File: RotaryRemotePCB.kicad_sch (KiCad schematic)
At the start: 10 parts, among them J1 Conn_01x02, J2 UART, J3 i2c, J4 Neopixel Connector, J5 EncoderRotary, J6 EncoderSwitch, SW1 RotaryEncoder_Switch, U1 TP4056, U2 WeMos_D1_mini

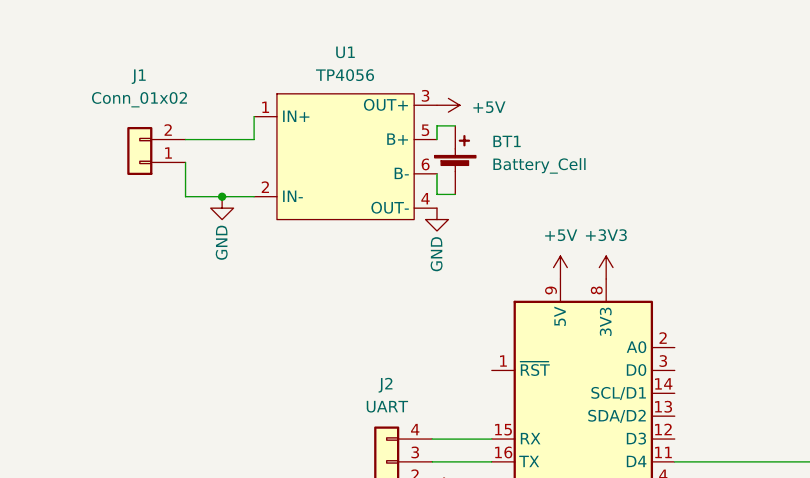
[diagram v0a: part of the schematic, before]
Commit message: Add git submodule
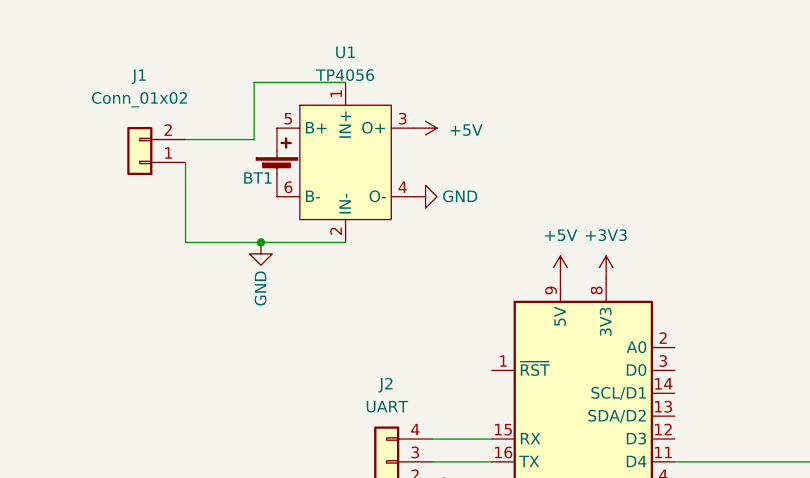
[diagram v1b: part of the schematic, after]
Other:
- moved on the sheet: BT1, U1
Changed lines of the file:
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@@
   (junction (at 205.994 86.106) (diameter 0) (color 0 0 0 0)
   )
+  (junction (at 135.128 56.642) (diameter 0) (color 0 0 0 0)
+  )
   (junction (at 230.632 86.106) (diameter 0) (color 0 0 0 0)
   )
@@
   (junction (at 230.632 91.186) (diameter 0) (color 0 0 0 0)
   )
-  (junction (at 130.81 51.562) (diameter 0) (color 0 0 0 0)
-  )
   (junction (at 205.994 91.186) (diameter 0) (color 0 0 0 0)
   )
+  (wire (pts (xy 135.128 56.642) (xy 126.746 56.642))
+    (stroke (width 0) (type default) (color 0 0 0 0))
+  )
   (wire (pts (xy 205.994 91.186) (xy 213.614 91.186))
     (stroke (width 0) (type default) (color 0 0 0 0))
@@
     (stroke (width 0) (type default) (color 0 0 0 0))
   )
-  (wire (pts (xy 154.686 43.688) (xy 156.718 43.688))
-    (stroke (width 0) (type default) (color 0 0 0 0))
-  )
   (wire (pts (xy 205.994 86.106) (xy 213.614 86.106))
     (stroke (width 0) (type default) (color 0 0 0 0))
@@
     (stroke (width 0) (type default) (color 0 0 0 0))
   )
-  (wire (pts (xy 126.746 51.562) (xy 126.746 47.752))
-    (stroke (width 0) (type default) (color 0 0 0 0))
-  )
   (wire (pts (xy 154.178 78.486) (xy 160.782 78.486))
     (stroke (width 0) (type default) (color 0 0 0 0))
@@
     (stroke (width 0) (type default) (color 0 0 0 0))
   )
-  (wire (pts (xy 154.686 49.022) (xy 154.686 51.308))
-    (stroke (width 0) (type default) (color 0 0 0 0))
-  )
-  (wire (pts (xy 154.686 45.212) (xy 154.686 43.688))
-    (stroke (width 0) (type default) (color 0 0 0 0))
-  )
   (wire (pts (xy 228.854 86.106) (xy 230.632 86.106))
     (stroke (width 0) (type default) (color 0 0 0 0))
@@
     (stroke (width 0) (type default) (color 0 0 0 0))
   )
-  (wire (pts (xy 134.366 45.212) (xy 134.366 42.672))
+  (wire (pts (xy 134.366 38.862) (xy 134.366 45.212))
     (stroke (width 0) (type default) (color 0 0 0 0))
   )
@@
     (stroke (width 0) (type default) (color 0 0 0 0))
   )
-  (wire (pts (xy 154.686 51.308) (xy 156.718 51.308))
+  (wire (pts (xy 144.526 38.862) (xy 134.366 38.862))
     (stroke (width 0) (type default) (color 0 0 0 0))
   )
@@
     (stroke (width 0) (type default) (color 0 0 0 0))
   )
-  (wire (pts (xy 134.366 51.562) (xy 130.81 51.562))
-    (stroke (width 0) (type default) (color 0 0 0 0))
-  )
-  (wire (pts (xy 130.81 51.562) (xy 126.746 51.562))
+  (wire (pts (xy 144.526 56.642) (xy 135.128 56.642))
+    (stroke (width 0) (type default) (color 0 0 0 0))
+  )
+  (wire (pts (xy 126.746 47.752) (xy 126.746 56.642))
     (stroke (width 0) (type default) (color 0 0 0 0))
   )
@@
     )
   )
-  (symbol (lib_id "power:GND") (at 130.81 51.562 0) (unit 1)
-    (in_bom yes) (on_board yes)
-    (property "Reference" "#PWR0101" (id 0) (at 130.81 57.912 0)
-      (effects (font (size 1.27 1.27)) hide)
-    )
-    (property "Value" "GND" (id 1) (at 130.81 58.674 90)
-      (effects (font (size 1.27 1.27)) (justify left))
-    )
-    (property "Footprint" "" (id 2) (at 130.81 51.562 0)
-      (effects (font (size 1.27 1.27)) hide)
-    )
-    (property "Datasheet" "" (id 3) (at 130.81 51.562 0)
+  (symbol (lib_id "power:GND") (at 135.128 56.642 0) (unit 1)
+    (in_bom yes) (on_board yes)
+    (property "Reference" "#PWR0101" (id 0) (at 135.128 62.992 0)
+      (effects (font (size 1.27 1.27)) hide)
+    )
+    (property "Value" "GND" (id 1) (at 135.128 63.754 90)
+      (effects (font (size 1.27 1.27)) (justify left))
+    )
+    (property "Footprint" "" (id 2) (at 135.128 56.642 0)
+      (effects (font (size 1.27 1.27)) hide)
+    )
+    (property "Datasheet" "" (id 3) (at 135.128 56.642 0)
       (effects (font (size 1.27 1.27)) hide)
     )
@@
     (pin "1")
   )
-  (symbol (lib_id "power:+5V") (at 154.686 41.402 270) (unit 1)
-    (in_bom yes) (on_board yes)
-    (property "Reference" "#PWR0106" (id 0) (at 150.876 41.402 0)
-      (effects (font (size 1.27 1.27)) hide)
-    )
-    (property "Value" "+5V" (id 1) (at 162.306 41.656 90)
+  (symbol (lib_id "power:+5V") (at 152.146 43.942 270) (unit 1)
+    (in_bom yes) (on_board yes)
+    (property "Reference" "#PWR0106" (id 0) (at 148.336 43.942 0)
+      (effects (font (size 1.27 1.27)) hide)
+    )
+    (property "Value" "+5V" (id 1) (at 159.766 44.196 90)
       (effects (font (size 1.27 1.27)) (justify right))
     )
-    (property "Footprint" "" (id 2) (at 154.686 41.402 0)
-      (effects (font (size 1.27 1.27)) hide)
-    )
-    (property "Datasheet" "" (id 3) (at 154.686 41.402 0)
+    (property "Footprint" "" (id 2) (at 152.146 43.942 0)
+      (effects (font (size 1.27 1.27)) hide)
+    )
+    (property "Datasheet" "" (id 3) (at 152.146 43.942 0)
       (effects (font (size 1.27 1.27)) hide)
     )
@@
     (pin "4")
   )
-  (symbol (lib_id "power:GND") (at 154.686 52.832 0) (unit 1)
-    (in_bom yes) (on_board yes)
-    (property "Reference" "#PWR0102" (id 0) (at 154.686 59.182 0)
-      (effects (font (size 1.27 1.27)) hide)
-    )
-    (property "Value" "GND" (id 1) (at 154.686 59.944 90)
-      (effects (font (size 1.27 1.27)) (justify left))
-    )
-    (property "Footprint" "" (id 2) (at 154.686 52.832 0)
-      (effects (font (size 1.27 1.27)) hide)
-    )
-    (property "Datasheet" "" (id 3) (at 154.686 52.832 0)
-      (effects (font (size 1.27 1.27)) hide)
-    )
-    (pin "1")
-  )
-  (symbol (lib_id "Device:Battery_Cell") (at 156.718 48.768 0) (unit 1)
-    (in_bom yes) (on_board yes) (fields_autoplaced)
-    (property "Reference" "BT1" (id 0) (at 160.782 45.4659 0)
-      (effects (font (size 1.27 1.27)) (justify left))
-    )
-    (property "Value" "Battery_Cell" (id 1) (at 160.782 48.0059 0)
-      (effects (font (size 1.27 1.27)) (justify left))
-    )
-    (property "Footprint" "Connector_PinHeader_2.54mm:PinHeader_1x02_P2.54mm_Vertical" (id 2) (at 156.718 47.244 90)
-      (effects (font (size 1.27 1.27)) hide)
-    )
-    (property "Datasheet" "~" (id 3) (at 156.718 47.244 90)
-      (effects (font (size 1.27 1.27)) hide)
-    )
+  (symbol (lib_id "power:GND") (at 152.146 51.562 90) (unit 1)
+    (in_bom yes) (on_board yes)
+    (property "Reference" "#PWR0102" (id 0) (at 158.496 51.562 0)
+      (effects (font (size 1.27 1.27)) hide)
+    )
+    (property "Value" "GND" (id 1) (at 159.258 51.562 90)
+      (effects (font (size 1.27 1.27)) (justify left))
+    )
+    (property "Footprint" "" (id 2) (at 152.146 51.562 0)
+      (effects (font (size 1.27 1.27)) hide)
+    )
+    (property "Datasheet" "" (id 3) (at 152.146 51.562 0)
+      (effects (font (size 1.27 1.27)) hide)
+    )
+    (pin "1")
+  )
+  (symbol (lib_id "Device:Battery_Cell") (at 136.906 49.022 0) (unit 1)
+    (in_bom yes) (on_board yes)
+    (property "Reference" "BT1" (id 0) (at 133.096 49.53 0)
+      (effects (font (size 1.27 1.27)) (justify left))
+    )
+    (property "Value" "Battery_Cell" (id 1) (at 140.97 48.2599 0)
+      (effects (font (size 1.27 1.27)) (justify left) hide)
+    )
+    (property "Footprint" "Connector_PinHeader_2.54mm:PinHeader_1x02_P2.54mm_Vertical" (id 2) (at 136.906 47.498 90)
+      (effects (font (size 1.27 1.27)) hide)
+    )
+    (property "Datasheet" "~" (id 3) (at 136.906 47.498 90)
+      (effects (font (size 1.27 1.27)) hide)
+    )
